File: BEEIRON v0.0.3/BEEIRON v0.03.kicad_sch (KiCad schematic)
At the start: 3 parts, among them U1 Regulator, U2 ThermoMeter

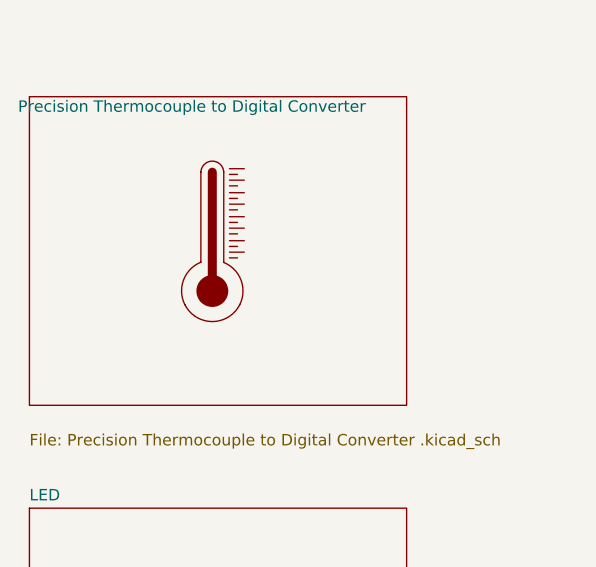
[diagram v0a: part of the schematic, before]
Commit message: added bakup file
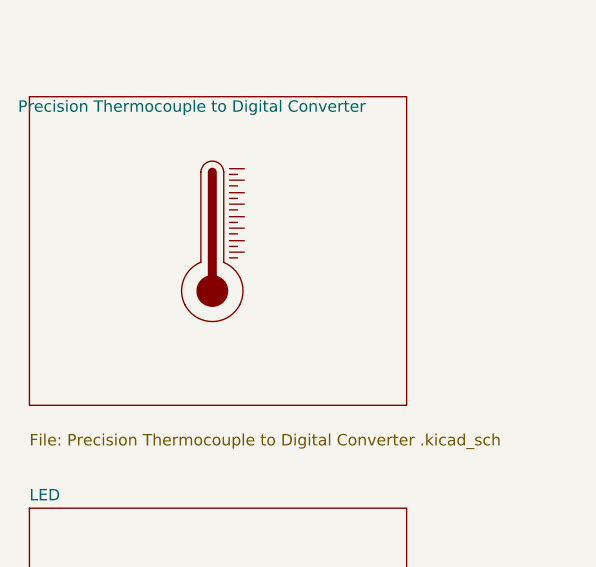
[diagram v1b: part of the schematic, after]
